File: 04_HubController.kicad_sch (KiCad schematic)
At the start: 79 parts, among them U11 CYUSB3304-68LTXx, Y1 26MHz

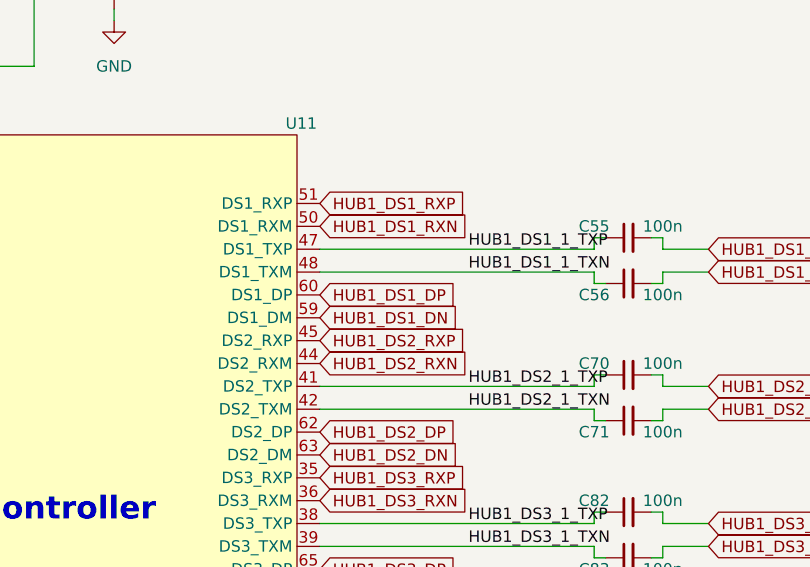
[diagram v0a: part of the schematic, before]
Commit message: settle on a layout
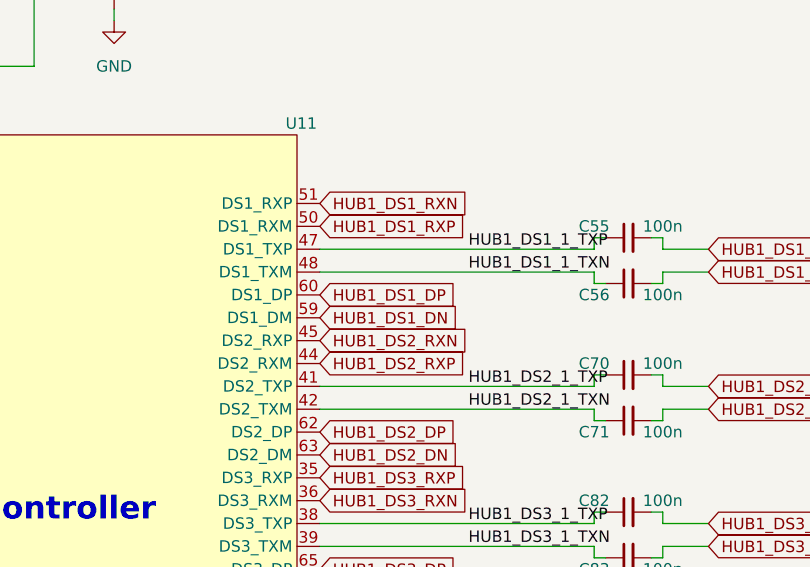
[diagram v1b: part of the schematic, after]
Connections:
- net HUB1_DS1_RXN: now also U11.51 (DS1_RXP); no longer U11.50 (DS1_RXM)
- net HUB1_DS1_RXP: now also U11.50 (DS1_RXM); no longer U11.51 (DS1_RXP)
- net HUB1_DS2_RXN: now also U11.45 (DS2_RXP); no longer U11.44 (DS2_RXM)
- net HUB1_DS2_RXP: now also U11.44 (DS2_RXM); no longer U11.45 (DS2_RXP)
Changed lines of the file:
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@@
-    )
-  )
-  (global_label "HUB1_DS1_RXN" (shape input) (at 224.79 53.34 0) (fields_autoplaced)
-    (effects (font (size 1.27 1.27)) (justify left))
-    (property "Intersheetrefs" "${INTERSHEET_REFS}" (at 242.3499 53.34 0)
-      (effects (font (size 1.27 1.27)) (justify left) hide)
     )
   )
@@
     )
   )
+  (global_label "HUB1_DS1_RXP" (shape input) (at 224.79 53.34 0) (fields_autoplaced)
+    (effects (font (size 1.27 1.27)) (justify left))
+    (property "Intersheetrefs" "${INTERSHEET_REFS}" (at 242.2894 53.34 0)
+      (effects (font (size 1.27 1.27)) (justify left) hide)
+    )
+  )
   (global_label "HUB1_DS1_DP" (shape input) (at 224.79 60.96 0) (fields_autoplaced)
     (effects (font (size 1.27 1.27)) (justify left))
     (property "Intersheetrefs" "${INTERSHEET_REFS}" (at 241.0799 60.96 0)
-      (effects (font (size 1.27 1.27)) (justify left) hide)
-    )
-  )
-  (global_label "HUB1_DS2_RXN" (shape input) (at 224.79 68.58 0) (fields_autoplaced)
-    (effects (font (size 1.27 1.27)) (justify left))
-    (property "Intersheetrefs" "${INTERSHEET_REFS}" (at 242.3499 68.58 0)
       (effects (font (size 1.27 1.27)) (justify left) hide)
     )
@@
     (property "Intersheetrefs" "${INTERSHEET_REFS}" (at 142.8834 53.34 0)
       (effects (font (size 1.27 1.27)) (justify right) hide)
+    )
+  )
+  (global_label "HUB1_DS1_RXN" (shape input) (at 224.79 50.8 0) (fields_autoplaced)
+    (effects (font (size 1.27 1.27)) (justify left))
+    (property "Intersheetrefs" "${INTERSHEET_REFS}" (at 242.3499 50.8 0)
+      (effects (font (size 1.27 1.27)) (justify left) hide)
+    )
+  )
+  (global_label "HUB1_DS2_RXP" (shape input) (at 224.79 68.58 0) (fields_autoplaced)
+    (effects (font (size 1.27 1.27)) (justify left))
+    (property "Intersheetrefs" "${INTERSHEET_REFS}" (at 242.2894 68.58 0)
+      (effects (font (size 1.27 1.27)) (justify left) hide)
     )
   )
@@
     )
   )
-  (global_label "HUB1_DS1_RXP" (shape input) (at 224.79 50.8 0) (fields_autoplaced)
-    (effects (font (size 1.27 1.27)) (justify left))
-    (property "Intersheetrefs" "${INTERSHEET_REFS}" (at 242.2894 50.8 0)
-      (effects (font (size 1.27 1.27)) (justify left) hide)
-    )
-  )
   (global_label "HUB1_DS2_DP" (shape input) (at 224.79 76.2 0) (fields_autoplaced)
     (effects (font (size 1.27 1.27)) (justify left))
@@
     (effects (font (size 1.27 1.27)) (justify left))
     (property "Intersheetrefs" "${INTERSHEET_REFS}" (at 285.2275 88.9 0)
+      (effects (font (size 1.27 1.27)) (justify left) hide)
+    )
+  )
+  (global_label "HUB1_DS2_RXN" (shape input) (at 224.79 66.04 0) (fields_autoplaced)
+    (effects (font (size 1.27 1.27)) (justify left))
+    (property "Intersheetrefs" "${INTERSHEET_REFS}" (at 242.3499 66.04 0)
       (effects (font (size 1.27 1.27)) (justify left) hide)
     )
@@
       (effects (font (size 1.27 1.27)) (justify left) hide)
     )
-  )
-  (global_label "HUB1_DS2_RXP" (shape input) (at 224.79 66.04 0) (fields_autoplaced)
-    (effects (font (size 1.27 1.27)) (justify left))
-    (property "Intersheetrefs" "${INTERSHEET_REFS}" (at 242.2894 66.04 0)
-      (effects (font (size 1.27 1.27)) (justify left) hide)
-    )

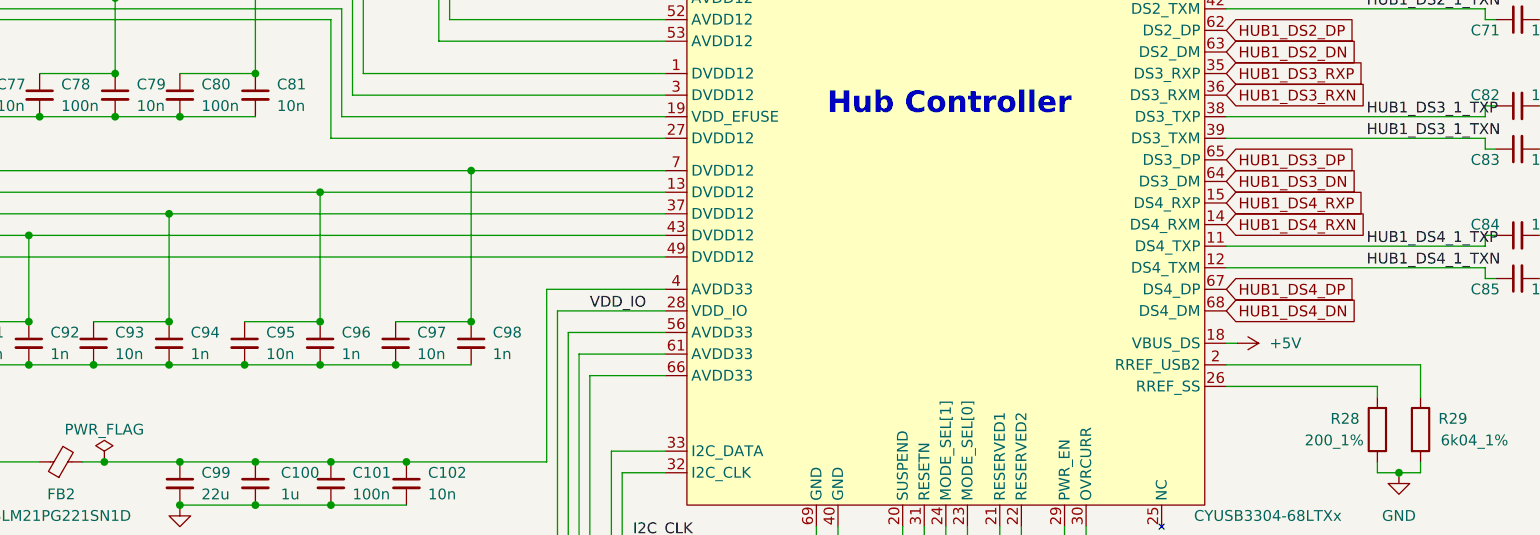
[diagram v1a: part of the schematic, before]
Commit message: finish layout draft
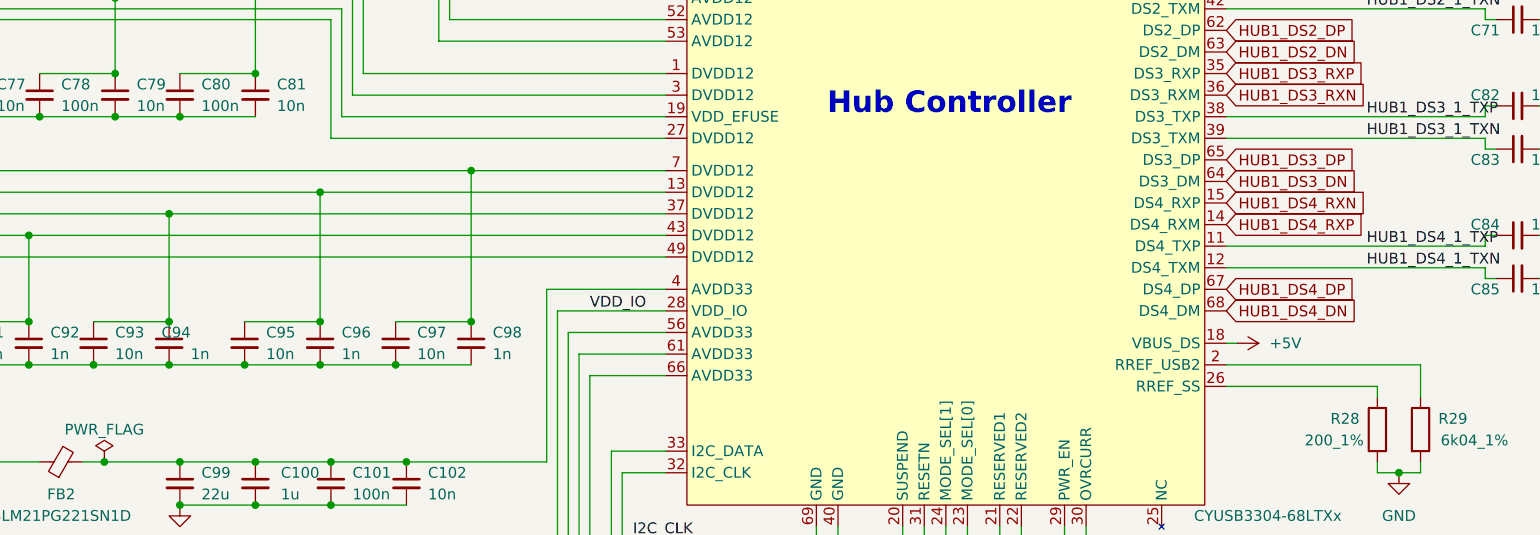
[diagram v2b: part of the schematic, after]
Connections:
- net HUB1_DS4_RXN: now also U11.15 (DS4_RXP); no longer U11.14 (DS4_RXM)
- net HUB1_DS4_RXP: now also U11.14 (DS4_RXM); no longer U11.15 (DS4_RXP)
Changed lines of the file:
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@@
-    )
-  )
-  (global_label "HUB1_DS4_RXN" (shape input) (at 224.79 99.06 0) (fields_autoplaced)
-    (effects (font (size 1.27 1.27)) (justify left))
-    (property "Intersheetrefs" "${INTERSHEET_REFS}" (at 242.3499 99.06 0)
-      (effects (font (size 1.27 1.27)) (justify left) hide)
     )
   )
@@
     )
   )
+  (global_label "HUB1_DS4_RXN" (shape input) (at 224.79 96.52 0) (fields_autoplaced)
+    (effects (font (size 1.27 1.27)) (justify left))
+    (property "Intersheetrefs" "${INTERSHEET_REFS}" (at 242.3499 96.52 0)
+      (effects (font (size 1.27 1.27)) (justify left) hide)
+    )
+  )
   (global_label "HUB1_DS4_DN" (shape input) (at 224.79 109.22 0) (fields_autoplaced)
     (effects (font (size 1.27 1.27)) (justify left))
@@
     )
   )
+  (global_label "HUB1_DS4_RXP" (shape input) (at 224.79 99.06 0) (fields_autoplaced)
+    (effects (font (size 1.27 1.27)) (justify left))
+    (property "Intersheetrefs" "${INTERSHEET_REFS}" (at 242.2894 99.06 0)
+      (effects (font (size 1.27 1.27)) (justify left) hide)
+    )
+  )
   (global_label "HUB1_DS3_RXN" (shape input) (at 224.79 83.82 0) (fields_autoplaced)
     (effects (font (size 1.27 1.27)) (justify left))
     (property "Intersheetrefs" "${INTERSHEET_REFS}" (at 242.3499 83.82 0)
-      (effects (font (size 1.27 1.27)) (justify left) hide)
-    )
-  )
-  (global_label "HUB1_DS4_RXP" (shape input) (at 224.79 96.52 0) (fields_autoplaced)
-    (effects (font (size 1.27 1.27)) (justify left))
-    (property "Intersheetrefs" "${INTERSHEET_REFS}" (at 242.2894 96.52 0)
       (effects (font (size 1.27 1.27)) (justify left) hide)
     )
@@
   )
   (symbol (lib_id "Device:C_Small") (at 100.33 113.03 0) (unit 1)
-    (in_bom yes) (on_board yes) (dnp no) (fields_autoplaced)
+    (in_bom yes) (on_board yes) (dnp no)
     (property "Reference" "C94" (at 102.87 111.7663 0)
-      (effects (font (size 1.27 1.27)) (justify left))
+      (effects (font (size 1.27 1.27)) (justify right))
     )
     (property "Value" "1n" (at 102.87 114.3063 0)

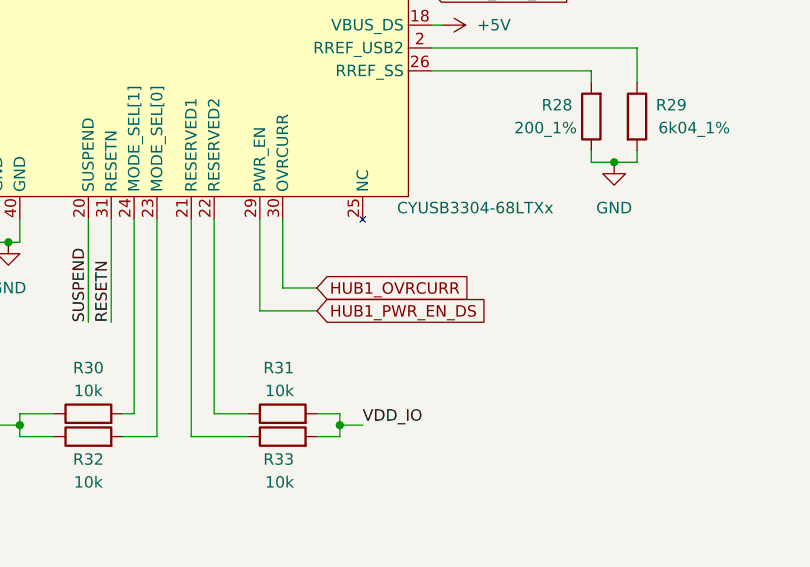
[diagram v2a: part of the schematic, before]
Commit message: fixing drcs
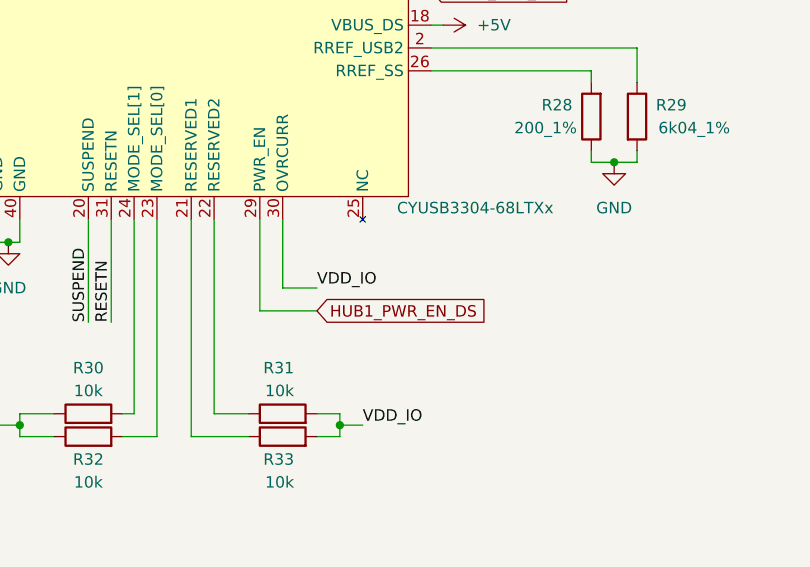
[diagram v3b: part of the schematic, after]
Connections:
- net HUB1_OVRCURR is gone; now on net +3V3: U11.30 (OVRCURR)
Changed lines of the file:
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@@
+    (effects (font (size 1.27 1.27)) (justify left bottom))
+  )
+  (label "VDD_IO" (at 212.09 142.24 0) (fields_autoplaced)
     (effects (font (size 1.27 1.27)) (justify left bottom))
   )
@@
       (effects (font (size 1.27 1.27)) (justify left) hide)
     )
-  )
-  (global_label "HUB1_OVRCURR" (shape input) (at 212.09 142.24 0) (fields_autoplaced)
-    (effects (font (size 1.27 1.27)) (justify left))
-    (property "Intersheetrefs" "${INTERSHEET_REFS}" (at 230.0129 142.24 0)
-      (effects (font (size 1.27 1.27)) (justify left) hide)
-    )
